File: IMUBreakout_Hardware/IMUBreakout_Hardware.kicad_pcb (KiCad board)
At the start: 2 copper layers, 6 parts, among them U1 Razor_9DOF_Sparkfun

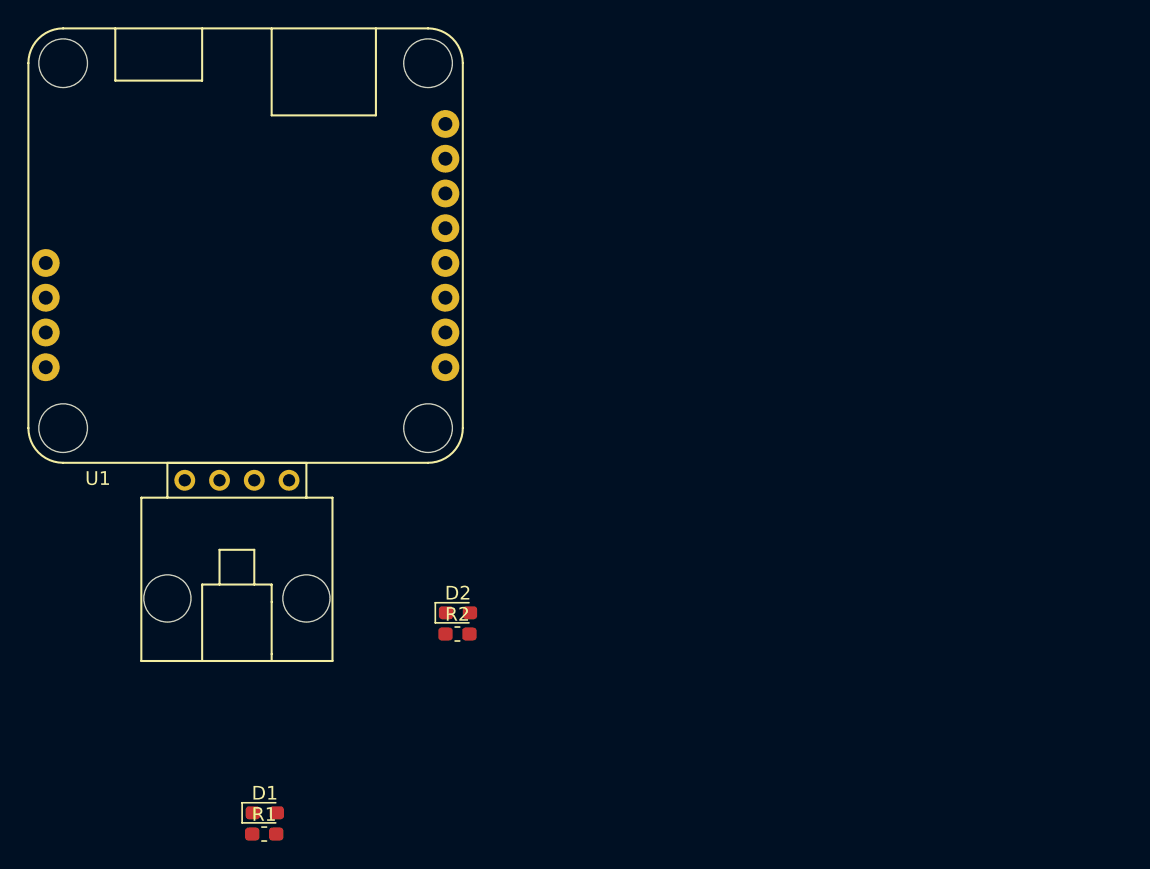
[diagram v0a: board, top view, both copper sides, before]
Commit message: PCB Finalzied and Made
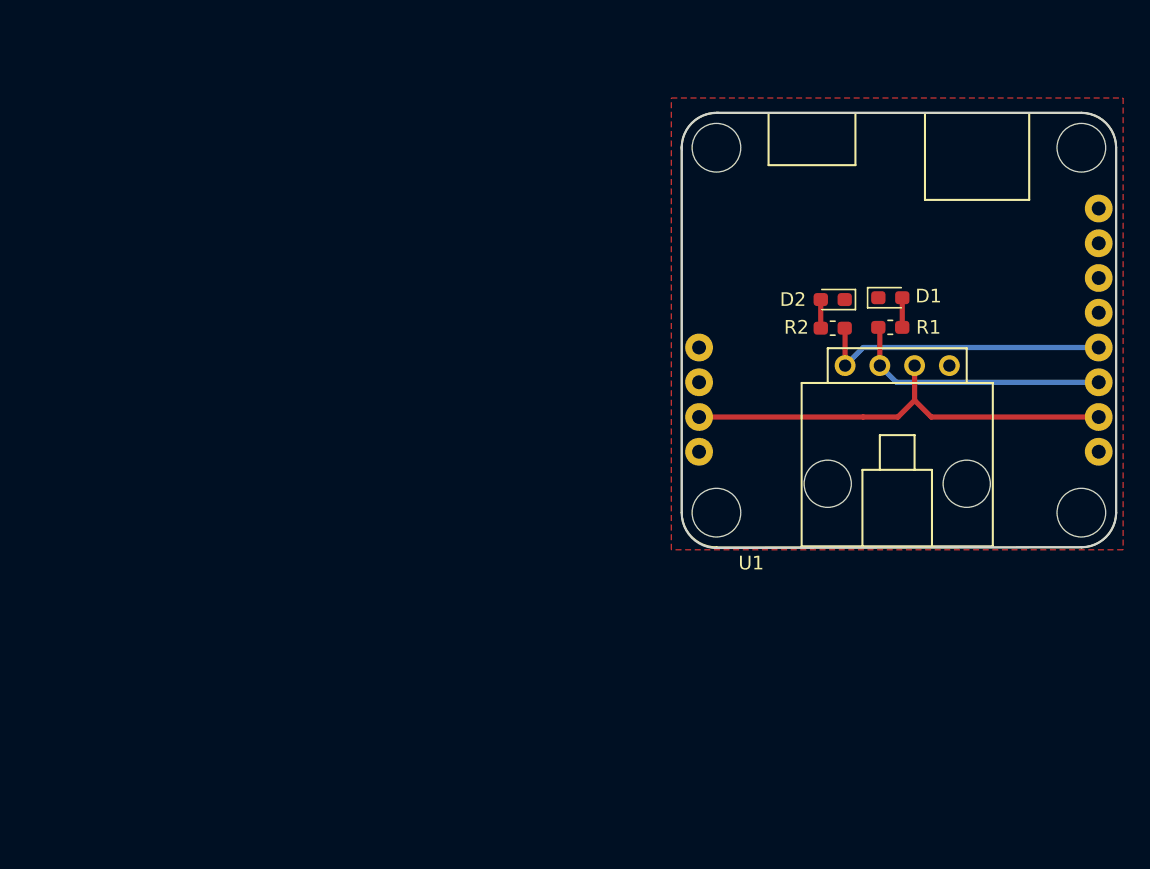
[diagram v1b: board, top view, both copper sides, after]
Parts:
- moved D1 59.2 mm to (160.8, 75.6)
- moved R1 58.9 mm to (160.8, 77.7), turned to 180 degrees
- moved Conn1 49.0 mm to (161.3, 80.5)
- moved U1 48.1 mm to (145.5, 93.8)
- moved D2 35.7 mm to (156.6, 75.7), turned to 180 degrees
- moved R2 35.4 mm to (156.6, 77.8)
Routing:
- net +3V3: track 0.00 -> 32.8 mm
- net TX: track 0.00 -> 21.8 mm
- net RX: track 0.00 -> 19.3 mm
- net Net-(D1-Pad2): track 0.00 -> 2.32 mm
- net Net-(D2-Pad2): track 0.00 -> 2.09 mm
- added copper zone on F.Cu, net GND
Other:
- board outline added: 31.8 x 31.8 mm
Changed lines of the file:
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@@
-(kicad_pcb (version 20171130) (host pcbnew "(5.0.2)-1")
+(kicad_pcb (version 20171130) (host pcbnew "(5.0.0)")
   (general
     (thickness 1.6)
-    (drawings 2)
-    (tracks 0)
+    (drawings 10)
+    (tracks 19)
     (zones 0)
     (modules 6)
@@
   )
   (setup
-    (last_trace_width 0.25)
+    (last_trace_width 0.381)
     (user_trace_width 0.381)
     (trace_clearance 0.2)
@@
   )
   (module MRDT_Connectors:MOLEX_SL_04_Horizontal (layer F.Cu)
-    (at 113.03 88.9 180)
-    (fp_text reference Conn1 (at -2.54 2.54 180) (layer F.SilkS) hide
+    (at 161.29 80.518 180)
+    (fp_text reference Conn1 (at -4.572 -2.032 180) (layer F.SilkS) hide
       (effects (font (size 1 1) (thickness 0.15)))
     )
@@
   )
   (module LED_SMD:LED_0603_1608Metric_Pad1.05x0.95mm_HandSolder (layer F.Cu)
-    (at 115.070001 113.205001)
+    (at 160.785626 75.55623)
     (descr "LED SMD 0603 (1608 Metric), square (rectangular) end terminal, IPC_7351 nominal, (Body size source: http://www.tortai-tech.com/upload/download/2011102023233369053.pdf), generated with kicad-footprint-generator")
     (tags "LED handsolder")
     (attr smd)
-    (fp_text reference D1 (at 0 -1.43) (layer F.SilkS)
+    (fp_text reference D1 (at 2.790374 -0.11823) (layer F.SilkS)
       (effects (font (size 1 1) (thickness 0.15)))
     )
@@
   )
   (module LED_SMD:LED_0603_1608Metric_Pad1.05x0.95mm_HandSolder (layer F.Cu)
-    (at 129.190001 98.585001)
+    (at 156.577 75.692 180)
     (descr "LED SMD 0603 (1608 Metric), square (rectangular) end terminal, IPC_7351 nominal, (Body size source: http://www.tortai-tech.com/upload/download/2011102023233369053.pdf), generated with kicad-footprint-generator")
     (tags "LED handsolder")
     (attr smd)
-    (fp_text reference D2 (at 0 -1.43) (layer F.SilkS)
-      (effects (font (size 1 1) (thickness 0.15)))
-    )
-    (fp_text value LED (at 0 1.43) (layer F.Fab)
+    (fp_text reference D2 (at 2.907 0 180) (layer F.SilkS)
+      (effects (font (size 1 1) (thickness 0.15)))
+    )
+    (fp_text value LED (at 0 1.43 180) (layer F.Fab)
       (effects (font (size 1 1) (thickness 0.15)))
     )
@@
     (fp_line (start 1.65 -0.73) (end 1.65 0.73) (layer F.CrtYd) (width 0.05))
     (fp_line (start 1.65 0.73) (end -1.65 0.73) (layer F.CrtYd) (width 0.05))
-    (fp_text user %R (at 0 0) (layer F.Fab)
+    (fp_text user %R (at 0 0 180) (layer F.Fab)
       (effects (font (size 0.4 0.4) (thickness 0.06)))
     )
-    (pad 1 smd roundrect (at -0.875 0) (size 1.05 0.95) (layers F.Cu F.Paste F.Mask) (roundrect_rratio 0.25)
+    (pad 1 smd roundrect (at -0.875 0 180) (size 1.05 0.95) (layers F.Cu F.Paste F.Mask) (roundrect_rratio 0.25)
       (net 1 GND))
-    (pad 2 smd roundrect (at 0.875 0) (size 1.05 0.95) (layers F.Cu F.Paste F.Mask) (roundrect_rratio 0.25)
+    (pad 2 smd roundrect (at 0.875 0 180) (size 1.05 0.95) (layers F.Cu F.Paste F.Mask) (roundrect_rratio 0.25)
       (net 6 "Net-(D2-Pad2)"))
     (model ${KISYS3DMOD}/LED_SMD.3dshapes/LED_0603_1608Metric.wrl
@@
   )
   (module Resistor_SMD:R_0603_1608Metric_Pad1.05x0.95mm_HandSolder (layer F.Cu)
-    (at 115.025001 114.755001)
+    (at 160.782 77.724 180)
     (descr "Resistor SMD 0603 (1608 Metric), square (rectangular) end terminal, IPC_7351 nominal with elongated pad for handsoldering. (Body size source: http://www.tortai-tech.com/upload/download/2011102023233369053.pdf), generated with kicad-footprint-generator")
     (tags "resistor handsolder")
     (attr smd)
-    (fp_text reference R1 (at 0 -1.43) (layer F.SilkS)
-      (effects (font (size 1 1) (thickness 0.15)))
-    )
-    (fp_text value 500 (at 0 1.43) (layer F.Fab)
-      (effects (font (size 1 1) (thickness 0.15)))
-    )
-    (fp_text user %R (at 0 0) (layer F.Fab)
+    (fp_text reference R1 (at -2.794 0 180) (layer F.SilkS)
+      (effects (font (size 1 1) (thickness 0.15)))
+    )
+    (fp_text value 500 (at 0 1.43 180) (layer F.Fab)
+      (effects (font (size 1 1) (thickness 0.15)))
+    )
+    (fp_text user %R (at 0 0 180) (layer F.Fab)
       (effects (font (size 0.4 0.4) (thickness 0.06)))
     )
@@
     (fp_line (start -0.8 -0.4) (end 0.8 -0.4) (layer F.Fab) (width 0.1))
     (fp_line (start -0.8 0.4) (end -0.8 -0.4) (layer F.Fab) (width 0.1))
-    (pad 2 smd roundrect (at 0.875 0) (size 1.05 0.95) (layers F.Cu F.Paste F.Mask) (roundrect_rratio 0.25)
+    (pad 2 smd roundrect (at 0.875 0 180) (size 1.05 0.95) (layers F.Cu F.Paste F.Mask) (roundrect_rratio 0.25)
       (net 4 RX))
-    (pad 1 smd roundrect (at -0.875 0) (size 1.05 0.95) (layers F.Cu F.Paste F.Mask) (roundrect_rratio 0.25)
+    (pad 1 smd roundrect (at -0.875 0 180) (size 1.05 0.95) (layers F.Cu F.Paste F.Mask) (roundrect_rratio 0.25)
       (net 5 "Net-(D1-Pad2)"))
     (model ${KISYS3DMOD}/Resistor_SMD.3dshapes/R_0603_1608Metric.wrl
@@
   )
   (module Resistor_SMD:R_0603_1608Metric_Pad1.05x0.95mm_HandSolder (layer F.Cu)
-    (at 129.145001 100.135001)
+    (at 156.577001 77.783001)
     (descr "Resistor SMD 0603 (1608 Metric), square (rectangular) end terminal, IPC_7351 nominal with elongated pad for handsoldering. (Body size source: http://www.tortai-tech.com/upload/download/2011102023233369053.pdf), generated with kicad-footprint-generator")
     (tags "resistor handsolder")
     (attr smd)
-    (fp_text reference R2 (at 0 -1.43) (layer F.SilkS)
+    (fp_text reference R2 (at -2.653001 -0.059001) (layer F.SilkS)
       (effects (font (size 1 1) (thickness 0.15)))
     )
@@
   )
   (module MRDT_Sensors:Razor_9DOF_Sparkfun (layer F.Cu)
-    (at 97.79 87.63)
+    (at 145.538 93.808185)
     (fp_text reference U1 (at 5.08 1.143) (layer F.SilkS)
       (effects (font (size 1 1) (thickness 0.15)))
@@
       (net 1 GND))
   )
+  (gr_line (start 148.082 62.0395) (end 174.752 62.0395) (layer Edge.Cuts) (width 0.15))
+  (gr_line (start 148.0185 93.853) (end 174.879 93.7895) (layer Edge.Cuts) (width 0.15))
+  (gr_arc (start 148.082 64.5795) (end 148.209 62.0395) (angle -97.04732902) (layer Edge.Cuts) (width 0.15))
+  (gr_arc (start 148.082 91.313) (end 145.542 91.313) (angle -90) (layer Edge.Cuts) (width 0.15))
+  (gr_arc (start 174.752 91.2495) (end 174.752 93.7895) (angle -90) (layer Edge.Cuts) (width 0.15))
+  (gr_line (start 177.292 64.5795) (end 177.292 91.3765) (layer Edge.Cuts) (width 0.15))
+  (gr_arc (start 174.752 64.5795) (end 177.292 64.5795) (angle -90) (layer Edge.Cuts) (width 0.15))
+  (gr_line (start 145.542 64.516) (end 145.542 91.2495) (layer Edge.Cuts) (width 0.15))
   (dimension 25.4 (width 0.3) (layer F.Fab)
     (gr_text "1.0000 in" (at 107.12 99.06 90) (layer F.Fab)
@@
     (arrow2b (pts (xy 134.62 127) (xy 135.746504 126.413579)))
   )
+  (segment (start 158.801999 84.276001) (end 146.808 84.276001) (width 0.381) (layer F.Cu) (net 2))
+  (segment (start 161.341999 84.276001) (end 158.801999 84.276001) (width 0.381) (layer F.Cu) (net 2))
+  (segment (start 162.56 80.518) (end 162.56 83.058) (width 0.381) (layer F.Cu) (net 2))
+  (segment (start 162.56 83.058) (end 161.341999 84.276001) (width 0.381) (layer F.Cu) (net 2))
+  (segment (start 163.778001 84.276001) (end 162.56 83.058) (width 0.381) (layer F.Cu) (net 2))
+  (segment (start 176.017999 84.276001) (end 163.778001 84.276001) (width 0.381) (layer F.Cu) (net 2))
+  (segment (start 157.48 77.811) (end 157.452001 77.783001) (width 0.381) (layer F.Cu) (net 3))
+  (segment (start 157.48 80.518) (end 157.48 77.811) (width 0.381) (layer F.Cu) (net 3))
+  (segment (start 158.801999 79.196001) (end 176.017999 79.196001) (width 0.381) (layer B.Cu) (net 3))
+  (segment (start 157.48 80.518) (end 158.801999 79.196001) (width 0.381) (layer B.Cu) (net 3))
+  (segment (start 160.02 77.837) (end 159.907 77.724) (width 0.381) (layer F.Cu) (net 4))
+  (segment (start 160.02 80.518) (end 160.02 77.837) (width 0.381) (layer F.Cu) (net 4))
+  (segment (start 161.238001 81.736001) (end 160.02 80.518) (width 0.381) (layer B.Cu) (net 4))
+  (segment (start 176.017999 81.736001) (end 161.238001 81.736001) (width 0.381) (layer B.Cu) (net 4))
+  (segment (start 161.556625 75.660231) (end 161.660626 75.55623) (width 0.381) (layer F.Cu) (net 5))
+  (segment (start 161.660626 77.720374) (end 161.657 77.724) (width 0.381) (layer F.Cu) (net 5))
+  (segment (start 161.660626 75.55623) (end 161.660626 77.720374) (width 0.381) (layer F.Cu) (net 5))
+  (segment (start 155.702 77.783) (end 155.702001 77.783001) (width 0.381) (layer F.Cu) (net 6))
+  (segment (start 155.702 75.692) (end 155.702 77.783) (width 0.381) (layer F.Cu) (net 6))
+  (zone (net 1) (net_name GND) (layer F.Cu) (hatch edge 0.508)
+    (connect_pads (clearance 0.508))
+    (min_thickness 0.254)
+    (fill yes (arc_segments 16) (thermal_gap 0.508) (thermal_bridge_width 0.508))
+    (polygon
+      (pts
+        (xy 144.78 60.96) (xy 177.8 60.96) (xy 177.8 93.98) (xy 144.78 93.98)
+      )
+    )
+  )
 )
